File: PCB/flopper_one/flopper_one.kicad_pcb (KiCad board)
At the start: 2 copper layers, 78 x 62 mm, 13 parts, among them J1 To PN532 ->, J2 <- ST7789, Q1 2N2219, SW1 SW_Omron_B3FS, SW2 SW_Omron_B3FS, SW3 SW_Omron_B3FS, SW4 SW_Omron_B3FS, SW5 SW_Omron_B3FS

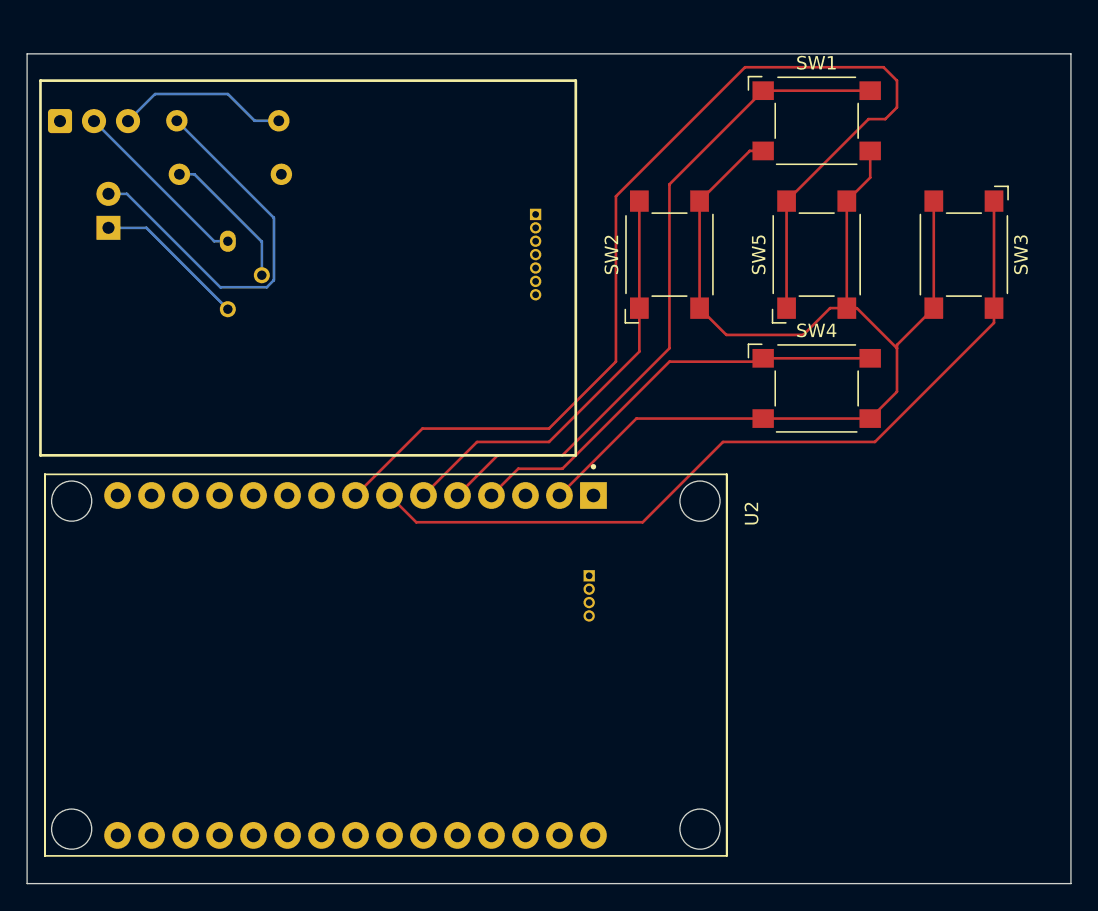
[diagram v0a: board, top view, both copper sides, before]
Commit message: routed the pcb
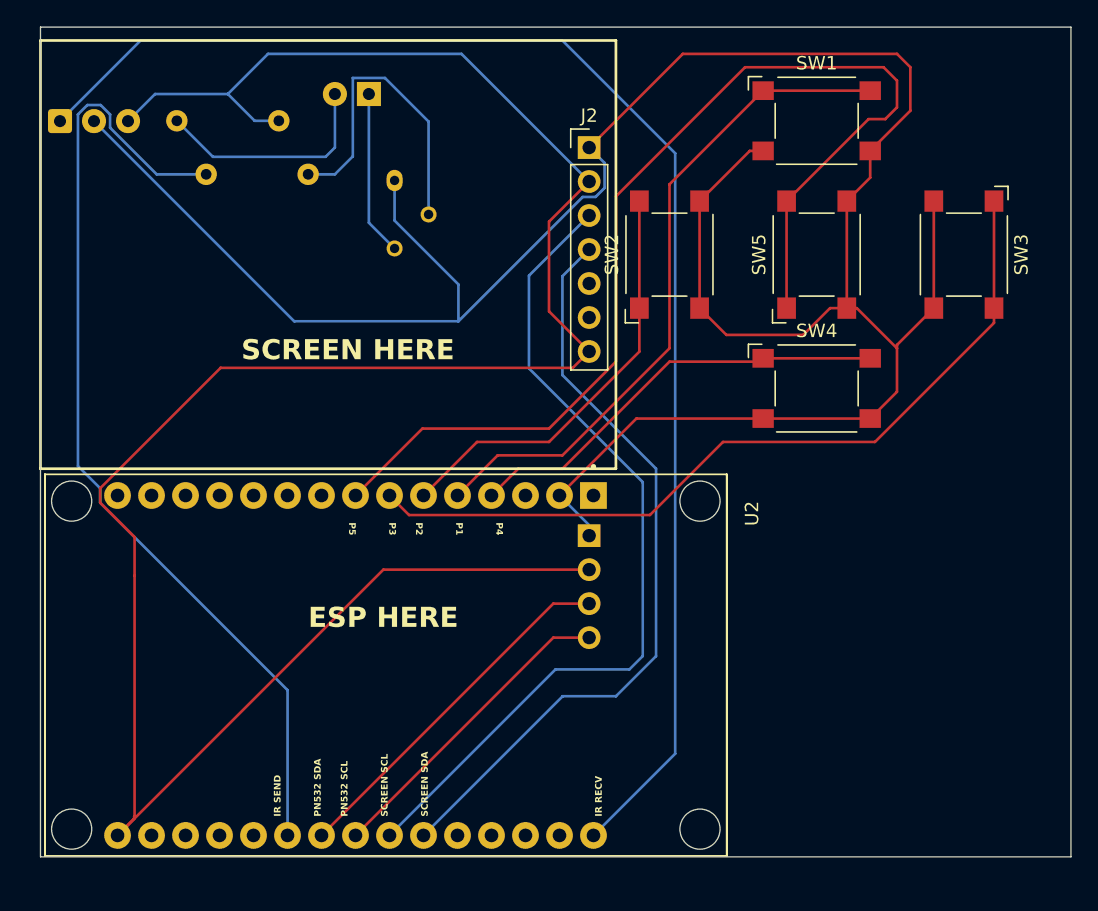
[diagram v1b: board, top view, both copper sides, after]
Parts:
- J1: footprint Connector_PinHeader_1.00mm:PinHeader_1x04_P1.00mm_Vertical -> Connector_PinHeader_2.54mm:PinHeader_1x04_P2.54mm_Vertical
- J2: footprint Connector_PinHeader_1.00mm:PinHeader_1x07_P1.00mm_Vertical -> Connector_PinHeader_2.54mm:PinHeader_1x07_P2.54mm_Vertical; moved to F.Cu
- moved D1 21.9 mm to (168.5, 65.0), turned to 180 degrees
- moved Q1 13.3 mm to (170.5, 71.5)
- moved R2 9.62 mm to (164.0, 71.0), turned to 180 degrees
- moved J2 6.40 mm to (185.0, 69.0), turned to 0 degrees
- moved J1 3.00 mm to (185.0, 98.0)
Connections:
- net Net-(U2-GPIO12) renamed /P4
- net Net-(U2-GPIO14) renamed /P1
- net Net-(U2-GPIO25) renamed /P5
- net Net-(U2-GPIO26) renamed /P3
- net Net-(U2-GPIO27) renamed /P2
- J1 pad 3: /SDA -> /SDA1
- J1 pad 4: /SCL -> /SCL1
- J2 pad 3: /SCL -> /SCL2
- J2 pad 4: /SDA -> /SDA2
- U2 pad 22: /SDA -> /SDA1
- U2 pad 23: /SCL -> /SCL1
- U2 pad 24: /SCL -> /SCL2
- U2 pad 25: /SDA -> /SDA2
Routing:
- net /VCC: track 12.9 -> 172.1 mm
- net Net-(U2-GPIO23): track 0.00 -> 105.5 mm
- net GND: track 102.0 -> 191.4 mm
- net Net-(U2-GPIO16): track 0.00 -> 73.0 mm
- net /SCL2: track 0.00 -> 62.8 mm
- net /SDA2: track 0.00 -> 57.1 mm
- net /SDA1: track 0.00 -> 27.2 mm
- net /SCL1: track 0.00 -> 23.6 mm
- net Net-(D1-A): track 30.4 -> 17.2 mm
- net Net-(Q1-B): track 10.8 -> 23.7 mm
- net Net-(D1-K): track 11.4 -> 12.3 mm
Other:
- board size 78 x 62 mm -> 77 x 62 mm
- board text added: "ESP HERE"
- board text added: "IR RECV"
- board text added: "IR SEND"
- board text added: "P1"
- board text added: "P2"
- board text added: "P3"
- board text added: "P4"
- board text added: "P5"
- board text added: "PN532 HERE"
- board text added: "PN532 SCL"
- board text added: "PN532 SDA"
- board text added: "SCREEN HERE"
- board text added: "SCREEN SCL"
- board text added: "SCREEN SDA"
